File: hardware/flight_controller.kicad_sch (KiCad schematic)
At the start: 77 parts, among them IC2 STM32F722RET6, IC3 W25Q128JVSIQ, J1 Conn_01x03, J2 JST SM08B-SRSS-TB(LF)(SN), J3 Conn_01x04, J4 Conn_01x04, J5 Conn_01x04, J6 USB4105-GF-A-060, Q1 TPRT9013-33GB, SW2 KMR221GLFS, U1 BMP581, U2 MP9943GQ-Z, U3 USBLC6-2P6, U4 MP9943GQ-Z, Y2 X322525MOB4SI

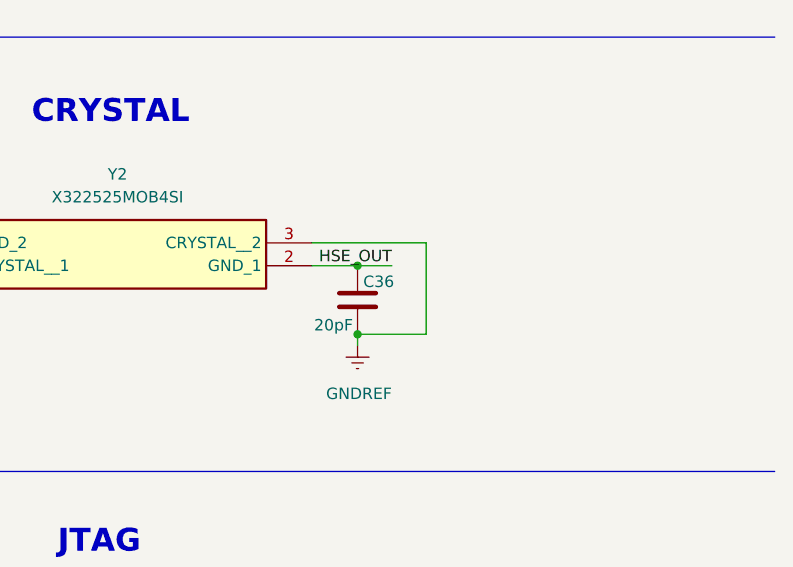
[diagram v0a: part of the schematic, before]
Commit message: crystal oscillator
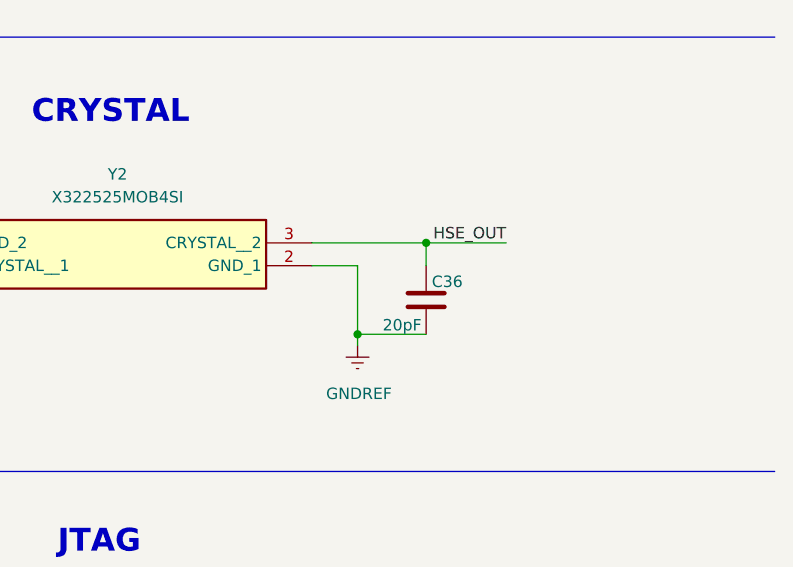
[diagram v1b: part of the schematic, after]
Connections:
- net GND: now also Y2.2 (GND_1); no longer Y2.3 (CRYSTAL__2)
- net HSE_OUT: now also Y2.3 (CRYSTAL__2); no longer Y2.2 (GND_1)
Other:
- moved on the sheet: C36
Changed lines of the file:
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@@
 	)
 	(junction
-		(at 424.18 193.04)
-		(diameter 0)
-		(color 0 0 0 0)
-	)
-	(junction
 		(at 314.96 163.83)
 		(diameter 0)
@@
 	)
 	(junction
+		(at 431.8 190.5)
+		(diameter 0)
+		(color 0 0 0 0)
+	)
+	(junction
 		(at 36.83 248.92)
 		(diameter 0)
@@
 	(wire
 		(pts
-			(xy 424.18 201.93) (xy 424.18 200.66)
-		)
-		(stroke
-			(width 0)
-			(type default)
-		)
-	)
-	(wire
-		(pts
 			(xy 33.02 185.42) (xy 38.1 185.42)
 		)
@@
 	(wire
 		(pts
+			(xy 424.18 200.66) (xy 431.8 200.66)
+		)
+		(stroke
+			(width 0)
+			(type default)
+		)
+	)
+	(wire
+		(pts
 			(xy 372.11 201.93) (xy 372.11 200.66)
 		)
@@
 	(wire
 		(pts
+			(xy 424.18 193.04) (xy 424.18 200.66)
+		)
+		(stroke
+			(width 0)
+			(type default)
+		)
+	)
+	(wire
+		(pts
 			(xy 92.71 33.02) (xy 96.52 33.02)
 		)
@@
 	(wire
 		(pts
+			(xy 419.1 193.04) (xy 424.18 193.04)
+		)
+		(stroke
+			(width 0)
+			(type default)
+		)
+	)
+	(wire
+		(pts
 			(xy 233.68 250.19) (xy 252.73 250.19)
 		)
@@
 	(wire
 		(pts
+			(xy 431.8 190.5) (xy 440.69 190.5)
+		)
+		(stroke
+			(width 0)
+			(type default)
+		)
+	)
+	(wire
+		(pts
 			(xy 57.15 130.81) (xy 100.33 130.81)
 		)
@@
 	(wire
 		(pts
-			(xy 419.1 193.04) (xy 424.18 193.04)
-		)
-		(stroke
-			(width 0)
-			(type default)
-		)
-	)
-	(wire
-		(pts
 			(xy 325.12 114.3) (xy 340.36 114.3)
 		)
@@
 	(wire
 		(pts
-			(xy 431.8 190.5) (xy 431.8 200.66)
+			(xy 431.8 190.5) (xy 431.8 193.04)
 		)
 		(stroke
@@
 	(wire
 		(pts
-			(xy 431.8 200.66) (xy 424.18 200.66)
-		)
-		(stroke
-			(width 0)
-			(type default)
-		)
-	)
-	(wire
-		(pts
 			(xy 369.57 111.76) (xy 382.27 111.76)
 		)
@@
 	(wire
 		(pts
-			(xy 424.18 193.04) (xy 427.99 193.04)
-		)
-		(stroke
-			(width 0)
-			(type default)
-		)
-	)
-	(wire
-		(pts
 			(xy 90.17 110.49) (xy 90.17 111.76)
 		)
@@
 	(wire
 		(pts
+			(xy 424.18 200.66) (xy 424.18 201.93)
+		)
+		(stroke
+			(width 0)
+			(type default)
+		)
+	)
+	(wire
+		(pts
 			(xy 281.94 58.42) (xy 278.13 58.42)
 		)
@@
 		)
 	)
+	(label "HSE_OUT"
+		(at 440.69 190.5 180)
+		(effects
+			(font
+				(size 1.27 1.27)
+			)
+			(justify right bottom)
+		)
+	)
 	(label "ESC_USART_RX"
 		(at 198.12 124.46 180)
@@
 		)
 	)
-	(label "HSE_OUT"
-		(at 427.99 193.04 180)
-		(effects
-			(font
-				(size 1.27 1.27)
-			)
-			(justify right bottom)
-		)
-	)
 	(label "USB_DN"
 		(at 22.86 49.53 0)
@@
 	(symbol
 		(lib_id "Device:C")
-		(at 424.18 196.85 180)
+		(at 431.8 196.85 180)
 		(unit 1)
 		(exclude_from_sim no)
@@
 		(dnp no)
 		(property "Reference" "C36"
-			(at 428.244 194.818 0)
+			(at 435.864 194.818 0)
 			(effects
 				(font
@@
 		)
 		(property "Value" "20pF"
-			(at 423.672 199.644 0)
+			(at 431.292 199.644 0)
 			(effects
 				(font
@@
 		)
 		(property "Footprint" "Capacitor_SMD:C_0402_1005Metric"
-			(at 423.2148 193.04 0)
+			(at 430.8348 193.04 0)
 			(effects
 				(font
@@
 		)
 		(property "Datasheet" "~"
-			(at 424.18 196.85 0)
+			(at 431.8 196.85 0)
 			(effects
 				(font
@@
 		)
 		(property "Description" "Unpolarized capacitor"
-			(at 424.18 196.85 0)
+			(at 431.8 196.85 0)
 			(effects
 				(font
